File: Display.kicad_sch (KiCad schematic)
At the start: 0 parts

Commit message: Updated pin assignments
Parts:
- added DS1: HDSP-A22C, DIPS1524W51P254L2520H725Q18N, symbol UTSVT_LeaderSOM:HDSP-A22C
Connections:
- new net DISP_A: DS1.12 (1A/2A_CATHODE)
- new net DISP_B: DS1.10 (1B/2B_CATHODE)
- new net DISP_C: DS1.9 (1C/2C_CATHODE)
- new net DISP_D: DS1.7 (1D/2D_CATHODE)
- new net DISP_E: DS1.1 (1E/2E_CATHODE)
- new net DISP_F: DS1.18 (1F/2F_CATHODE)
- new net DISP_G: DS1.15 (1G/2G_CATHODE)
- new net DISP_H: DS1.14 (1H/2H_CATHODE)
- new net DISP_J: DS1.6 (1J/2J_CATHODE)
- new net DISP_K: DS1.5 (1K/2K_CATHODE)
- new net DISP_L: DS1.4 (1L/2L_CATHODE)
- new net DISP_M: DS1.2 (1M/2M_CATHODE)
- new net DISP_N: DS1.13 (1N/2N_CATHODE)
- new net DISP_P: DS1.17 (1P/2P_CATHODE)
- new net GND: DS1.11 (DIGIT_NO._2_COMMON_ANODE), DS1.16 (DIGIT_NO._1_COMMON_ANODE)
- no-connect marks 0 -> 2
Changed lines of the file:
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@@
 (kicad_sch (version 20230121) (generator eeschema)
   (paper "A4")
+  (no_connect (at 116.84 105.41))
+  (no_connect (at 116.84 92.71))
+  (wire (pts (xy 182.88 105.41) (xy 198.12 105.41))
+    (stroke (width 0) (type default))
+  )
+  (wire (pts (xy 182.88 92.71) (xy 198.12 92.71))
+    (stroke (width 0) (type default))
+  )
+  (wire (pts (xy 198.12 105.41) (xy 198.12 106.045))
+    (stroke (width 0) (type default))
+  )
+  (wire (pts (xy 198.12 92.71) (xy 198.12 93.345))
+    (stroke (width 0) (type default))
+  )
+  (hierarchical_label "DISP_J" (shape input) (at 116.84 100.33 180) (fields_autoplaced)
+    (effects (font (size 1.27 1.27)) (justify right))
+  )
+  (hierarchical_label "DISP_E" (shape input) (at 116.84 87.63 180) (fields_autoplaced)
+    (effects (font (size 1.27 1.27)) (justify right))
+  )
+  (hierarchical_label "DISP_F" (shape input) (at 182.88 87.63 0) (fields_autoplaced)
+    (effects (font (size 1.27 1.27)) (justify left))
+  )
+  (hierarchical_label "DISP_B" (shape input) (at 182.88 107.95 0) (fields_autoplaced)
+    (effects (font (size 1.27 1.27)) (justify left))
+  )
+  (hierarchical_label "DISP_H" (shape input) (at 182.88 97.79 0) (fields_autoplaced)
+    (effects (font (size 1.27 1.27)) (justify left))
+  )
+  (hierarchical_label "DISP_D" (shape input) (at 116.84 102.87 180) (fields_autoplaced)
+    (effects (font (size 1.27 1.27)) (justify right))
+  )
+  (hierarchical_label "DISP_M" (shape input) (at 116.84 90.17 180) (fields_autoplaced)
+    (effects (font (size 1.27 1.27)) (justify right))
+  )
+  (hierarchical_label "DISP_L" (shape input) (at 116.84 95.25 180) (fields_autoplaced)
+    (effects (font (size 1.27 1.27)) (justify right))
+  )
+  (hierarchical_label "DISP_G" (shape input) (at 182.88 95.25 0) (fields_autoplaced)
+    (effects (font (size 1.27 1.27)) (justify left))
+  )
+  (hierarchical_label "DISP_P" (shape input) (at 182.88 90.17 0) (fields_autoplaced)
+    (effects (font (size 1.27 1.27)) (justify left))
+  )
+  (hierarchical_label "DISP_C" (shape input) (at 116.84 107.95 180) (fields_autoplaced)
+    (effects (font (size 1.27 1.27)) (justify right))
+  )
+  (hierarchical_label "DISP_N" (shape input) (at 182.88 100.33 0) (fields_autoplaced)
+    (effects (font (size 1.27 1.27)) (justify left))
+  )
+  (hierarchical_label "DISP_A" (shape input) (at 182.88 102.87 0) (fields_autoplaced)
+    (effects (font (size 1.27 1.27)) (justify left))
+  )
+  (hierarchical_label "DISP_K" (shape input) (at 116.84 97.79 180) (fields_autoplaced)
+    (effects (font (size 1.27 1.27)) (justify right))
+  )
+  (symbol (lib_id "UTSVT_LeaderSOM:HDSP-A22C") (at 116.84 87.63 0) (unit 1)
+    (in_bom yes) (on_board yes) (dnp no)
+    (property "Reference" "DS1" (at 149.86 80.645 0)
+      (effects (font (size 1.27 1.27)))
+    )
+    (property "Value" "HDSP-A22C" (at 149.86 83.185 0)
+      (effects (font (size 1.27 1.27)))
+    )
+    (property "Footprint" "DIPS1524W51P254L2520H725Q18N" (at 179.07 182.55 0)
+      (effects (font (size 1.27 1.27)) (justify left top) hide)
+    )
+    (property "Datasheet" "https://docs.broadcom.com/docs/HDSP-A2xC-DS" (at 179.07 282.55 0)
+      (effects (font (size 1.27 1.27)) (justify left top) hide)
+    )
+    (property "Height" "7.25" (at 179.07 482.55 0)
+      (effects (font (size 1.27 1.27)) (justify left top) hide)
+    )
+    (property "Mouser Part Number" "630-HDSP-A22C" (at 179.07 582.55 0)
+      (effects (font (size 1.27 1.27)) (justify left top) hide)
+    )
+    (property "Mouser Price/Stock" "https://www.mouser.co.uk/ProductDetail/Broadcom-Avago/HDSP-A22C?qs=mhB89zxvawkE7eTk4oWrWQ%3D%3D" (at 179.07 682.55 0)
+      (effects (font (size 1.27 1.27)) (justify left top) hide)
+    )
+    (property "Manufacturer_Name" "Avago Technologies" (at 179.07 782.55 0)
+      (effects (font (size 1.27 1.27)) (justify left top) hide)
+    )
+    (property "Manufacturer_Part_Number" "HDSP-A22C" (at 179.07 882.55 0)
+      (effects (font (size 1.27 1.27)) (justify left top) hide)
+    )
+    (pin "1")
+    (pin "10")
+    (pin "11")
+    (pin "12")
+    (pin "13")
+    (pin "14")
+    (pin "15")
+    (pin "16")
+    (pin "17")
+    (pin "18")
+    (pin "2")
+    (pin "3")
+    (pin "4")
+    (pin "5")
+    (pin "6")
+    (pin "7")
+    (pin "8")
+    (pin "9")
+    (instances
+      (project "LeaderSOM"
+        (path "/192d0c36-944e-4927-949b-263b8c85a7ca/48d44a6a-93f2-4d40-b0ae-ce24d0554ae2"
+          (reference "DS1") (unit 1)
+        )
+      )
+    )
+  )
+  (symbol (lib_id "power:GND") (at 198.12 106.045 0) (unit 1)
+    (in_bom yes) (on_board yes) (dnp no)
+    (property "Reference" "#PWR021" (at 198.12 112.395 0)
+      (effects (font (size 1.27 1.27)) hide)
+    )
+    (property "Value" "GND" (at 198.247 110.4392 0)
+      (effects (font (size 1.27 1.27)))
+    )
+    (property "Footprint" "" (at 198.12 106.045 0)
+      (effects (font (size 1.27 1.27)) hide)
+    )
+    (property "Datasheet" "" (at 198.12 106.045 0)
+      (effects (font (size 1.27 1.27)) hide)
+    )
+    (pin "1")
+    (instances
+      (project "LeaderSOM"
+        (path "/192d0c36-944e-4927-949b-263b8c85a7ca"
+          (reference "#PWR021") (unit 1)
+        )
+        (path "/192d0c36-944e-4927-949b-263b8c85a7ca/48d44a6a-93f2-4d40-b0ae-ce24d0554ae2"
+          (reference "#PWR027") (unit 1)
+        )
+      )
+      (project "BPS-Leader"
+        (path "/c248b171-df31-4e8a-afb6-607fa2df334b"
+          (reference "#PWR08") (unit 1)
+        )
+      )
+    )
+  )
+  (symbol (lib_id "power:GND") (at 198.12 93.345 0) (unit 1)
+    (in_bom yes) (on_board yes) (dnp no)
+    (property "Reference" "#PWR021" (at 198.12 99.695 0)
+      (effects (font (size 1.27 1.27)) hide)
+    )
+    (property "Value" "GND" (at 198.247 97.7392 0)
+      (effects (font (size 1.27 1.27)))
+    )
+    (property "Footprint" "" (at 198.12 93.345 0)
+      (effects (font (size 1.27 1.27)) hide)
+    )
+    (property "Datasheet" "" (at 198.12 93.345 0)
+      (effects (font (size 1.27 1.27)) hide)
+    )
+    (pin "1")
+    (instances
+      (project "LeaderSOM"
+        (path "/192d0c36-944e-4927-949b-263b8c85a7ca"
+          (reference "#PWR021") (unit 1)
+        )
+        (path "/192d0c36-944e-4927-949b-263b8c85a7ca/48d44a6a-93f2-4d40-b0ae-ce24d0554ae2"
+          (reference "#PWR028") (unit 1)
+        )
+      )
+      (project "BPS-Leader"
+        (path "/c248b171-df31-4e8a-afb6-607fa2df334b"
+          (reference "#PWR08") (unit 1)
+        )
+      )
+    )
+  )
 )

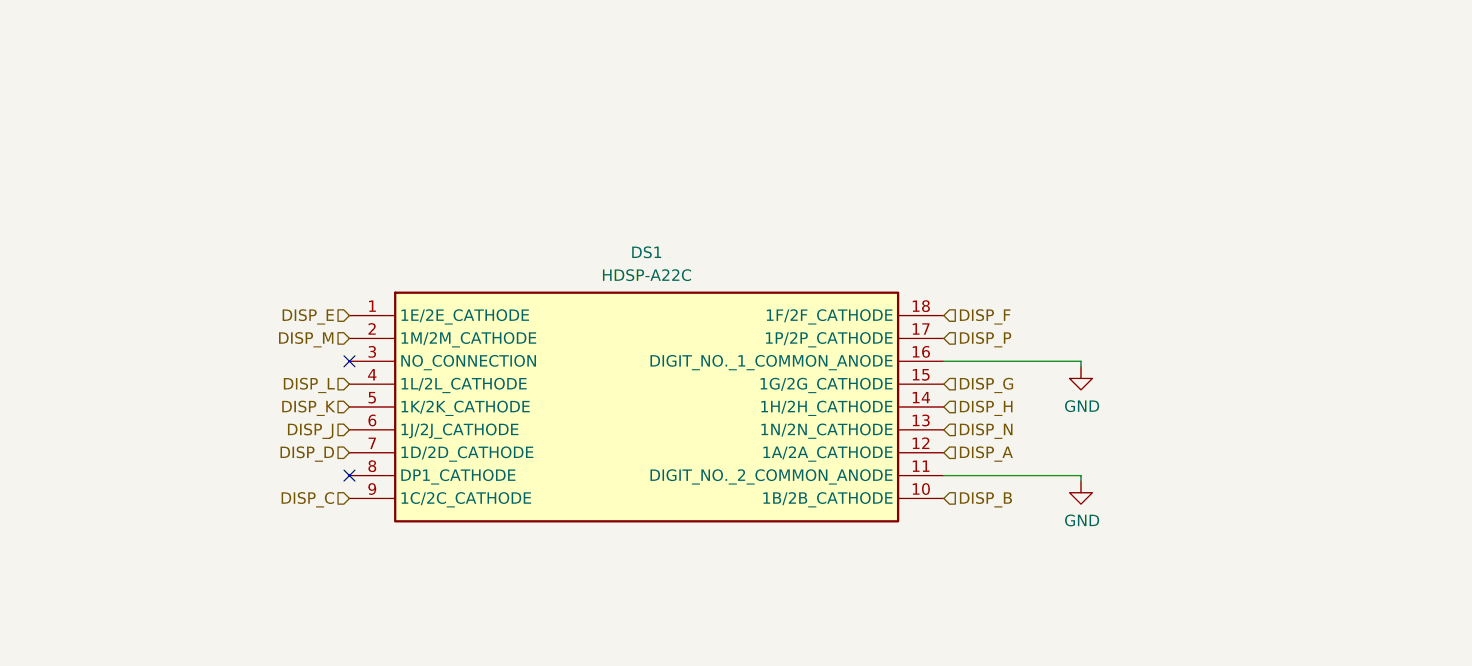
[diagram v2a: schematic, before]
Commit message: Updated power dist and CAN circuitry
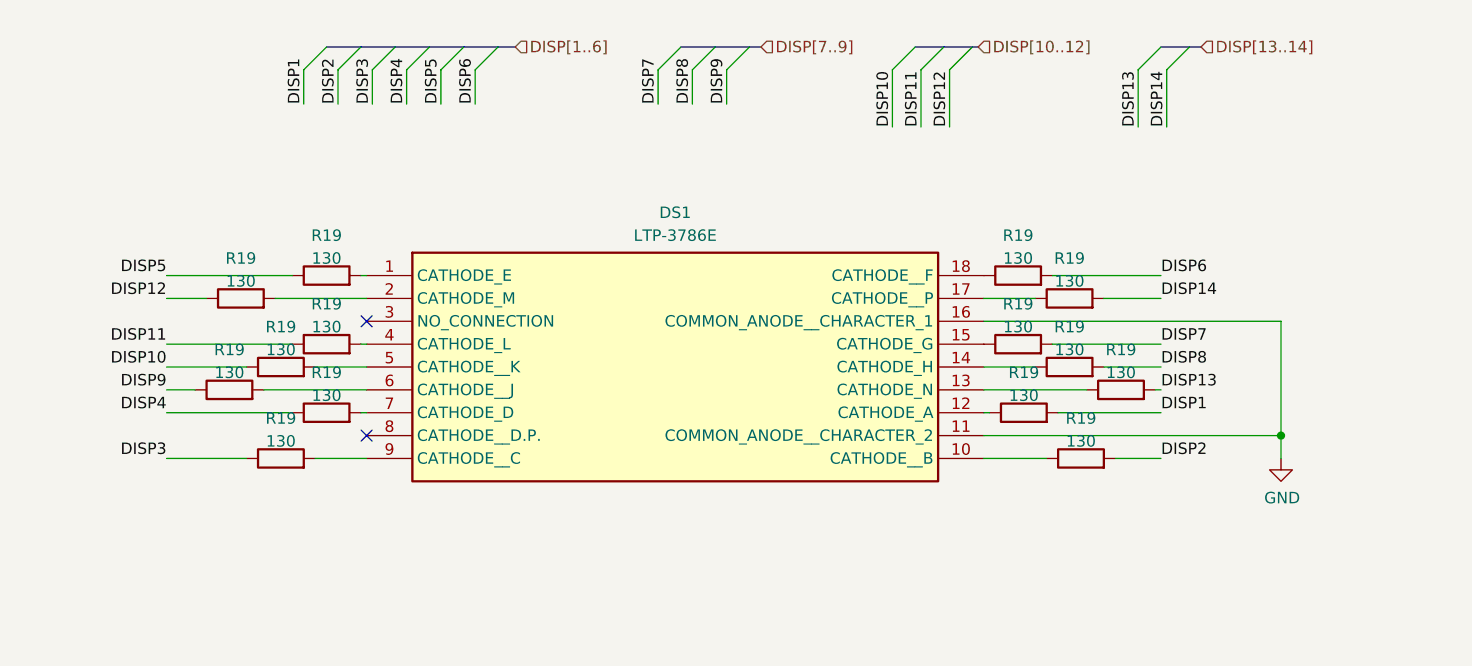
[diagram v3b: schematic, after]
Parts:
- removed DS1: HDSP-A22C, DIPS1524W51P254L2520H725Q18N, symbol UTSVT_LeaderSOM:HDSP-A22C
- added DS1: LTP-3786E, DIPS1499W50P254L2520H805Q18N, symbol UTSVT_LeaderSOM:LTP-3786E
- added R19 (x14): 130, Resistor_SMD:R_0805_2012Metric, symbol Device:R
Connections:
- net GND: now also DS1.11 (COMMON_ANODE__CHARACTER_2), DS1.16 (COMMON_ANODE__CHARACTER_1)
- new net: DS1.10 (CATHODE__B), R19.1
- new net: DS1.4 (CATHODE_L), R19.2
- new net: DS1.15 (CATHODE_G), R19.1
- new net: DS1.18 (CATHODE__F), R19.1
- new net: DS1.1 (CATHODE_E), R19.2
- new net: DS1.12 (CATHODE_A), R19.1
- new net: DS1.13 (CATHODE_N), R19.1
- new net: DS1.14 (CATHODE_H), R19.1
- new net: DS1.17 (CATHODE__P), R19.1
- new net: DS1.2 (CATHODE_M), R19.2
- new net: DS1.5 (CATHODE__K), R19.2
- new net: DS1.6 (CATHODE__J), R19.2
- new net: DS1.7 (CATHODE_D), R19.2
- new net: DS1.9 (CATHODE__C), R19.2
- new net DISP1: R19.2
- new net DISP10: R19.1
- new net DISP11: R19.1
- new net DISP12: R19.1
- new net DISP13: R19.2
- new net DISP14: R19.2
- new net DISP2: R19.2
- new net DISP3: R19.1
- new net DISP4: R19.1
- new net DISP5: R19.1
- new net DISP6: R19.2
- new net DISP7: R19.2
- new net DISP8: R19.2
- new net DISP9: R19.1

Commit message: Updated symbols
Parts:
- removed DS1: LTP-3786E, DIPS1499W50P254L2520H805Q18N, symbol UTSVT_LeaderSOM:LTP-3786E
- added DS1: LTP-3786E, DIPS1499W50P254L2520H805Q18N, symbol utsvt-misc:LTP-3786E
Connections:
- net GND: now also DS1.11 (COMMON_ANODE__CHARACTER_2), DS1.16 (COMMON_ANODE__CHARACTER_1)
- net at R19.1: now also DS1.10 (CATHODE__B)
- net at R19.2: now also DS1.4 (CATHODE_L)
- net at R19.1: now also DS1.15 (CATHODE_G)
- net at R19.1: now also DS1.18 (CATHODE__F)
- net at R19.2: now also DS1.1 (CATHODE_E)
- net at R19.1: now also DS1.12 (CATHODE_A)
- net at R19.1: now also DS1.13 (CATHODE_N)
- net at R19.1: now also DS1.14 (CATHODE_H)
- net at R19.1: now also DS1.17 (CATHODE__P)
- net at R19.2: now also DS1.2 (CATHODE_M)
- net at R19.2: now also DS1.5 (CATHODE__K)
- net at R19.2: now also DS1.6 (CATHODE__J)
- net at R19.2: now also DS1.7 (CATHODE_D)
- net at R19.2: now also DS1.9 (CATHODE__C)

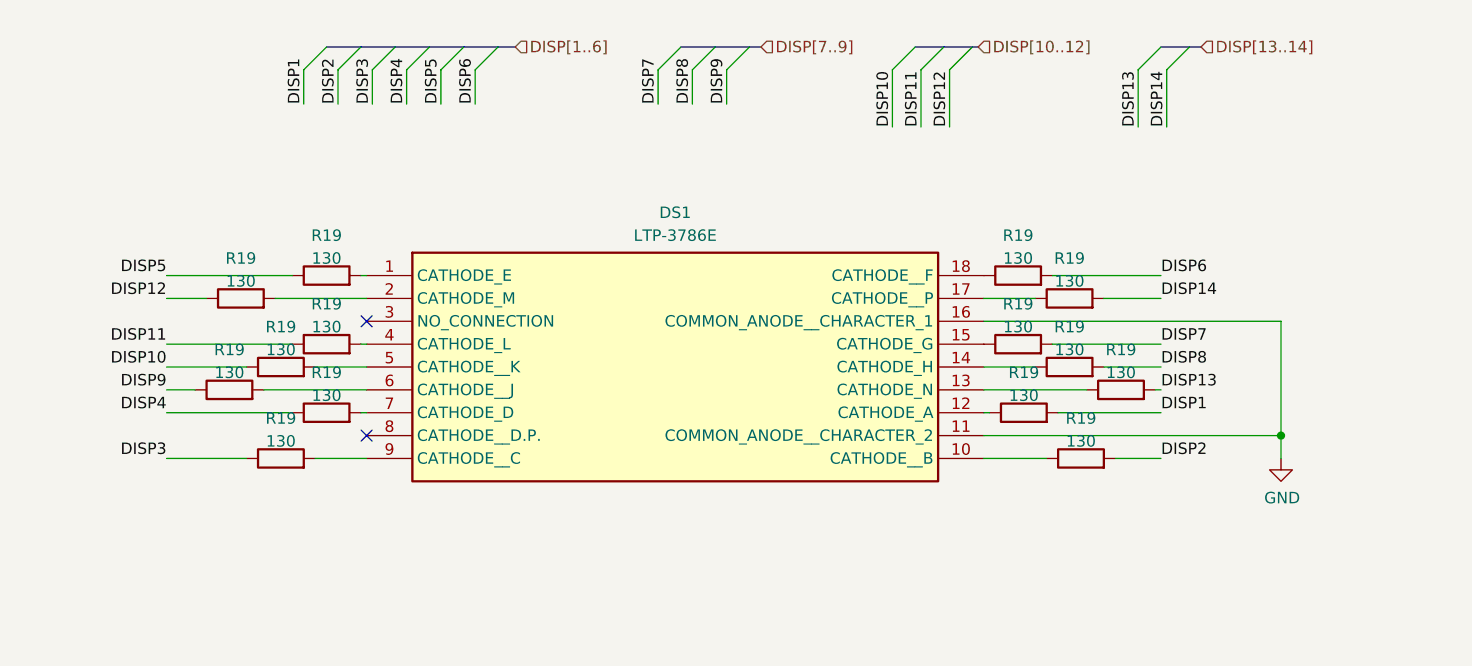
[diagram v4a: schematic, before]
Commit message: a
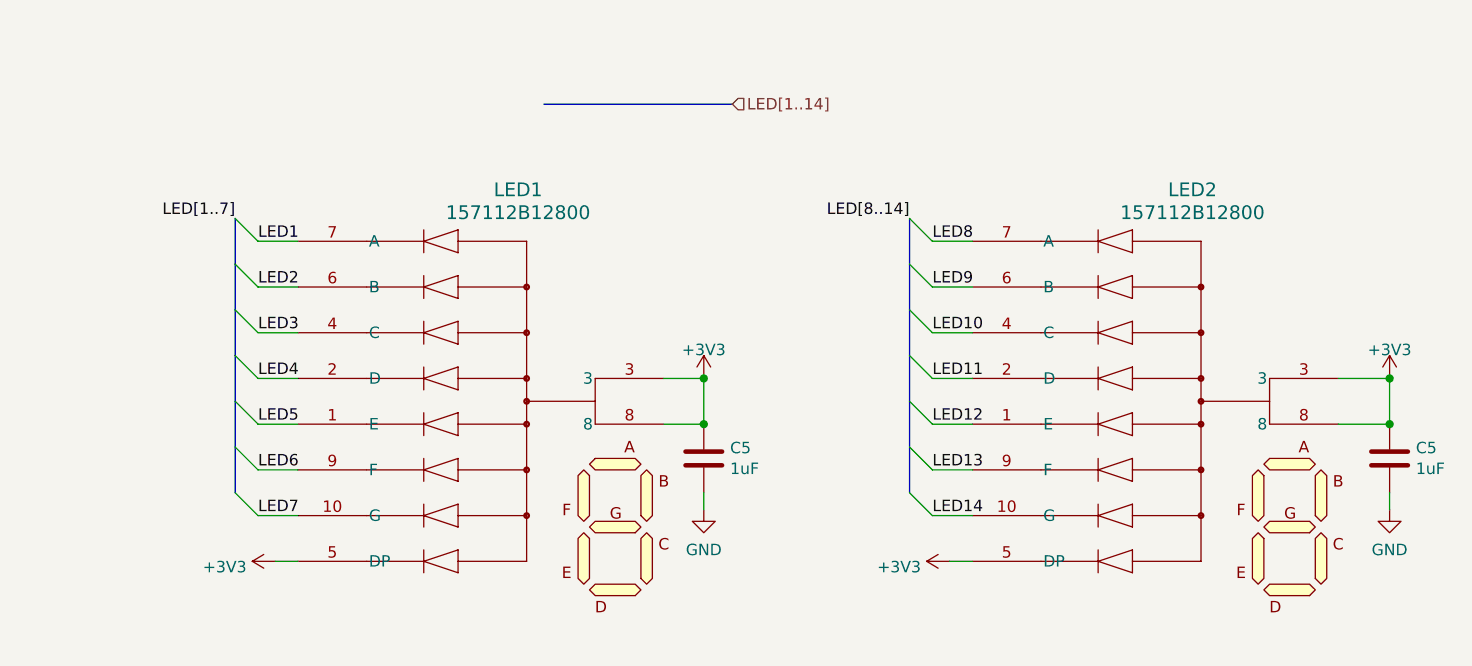
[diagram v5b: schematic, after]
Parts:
- removed DS1: LTP-3786E, DIPS1499W50P254L2520H805Q18N, symbol utsvt-misc:LTP-3786E
- removed R19 (x14): 130, Resistor_SMD:R_0805_2012Metric, symbol Device:R
- added C5 (x2): 1uF, Capacitor_SMD:C_0805_2012Metric, symbol Device:C
- added LED1, LED2: 157112B12800, UTSVT_Special:SMT_1S12800_WRE, symbol utsvt-misc:157112B12800
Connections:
- net GND: now also C5.2, C5.2
- new net +3V3: C5.1, C5.1, LED1.3, LED1.5 (DP), LED1.8, LED2.3, LED2.5 (DP), LED2.8
- new net LED1: LED1.7 (A)
- new net LED10: LED2.4 (C)
- new net LED11: LED2.2 (D)
- new net LED12: LED2.1 (E)
- new net LED13: LED2.9 (F)
- new net LED14: LED2.10 (G)
- new net LED2: LED1.6 (B)
- new net LED3: LED1.4 (C)
- new net LED4: LED1.2 (D)
- new net LED5: LED1.1 (E)
- new net LED6: LED1.9 (F)
- new net LED7: LED1.10 (G)
- new net LED8: LED2.7 (A)
- new net LED9: LED2.6 (B)
- no-connect marks 2 -> 0

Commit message: updated pin assignments
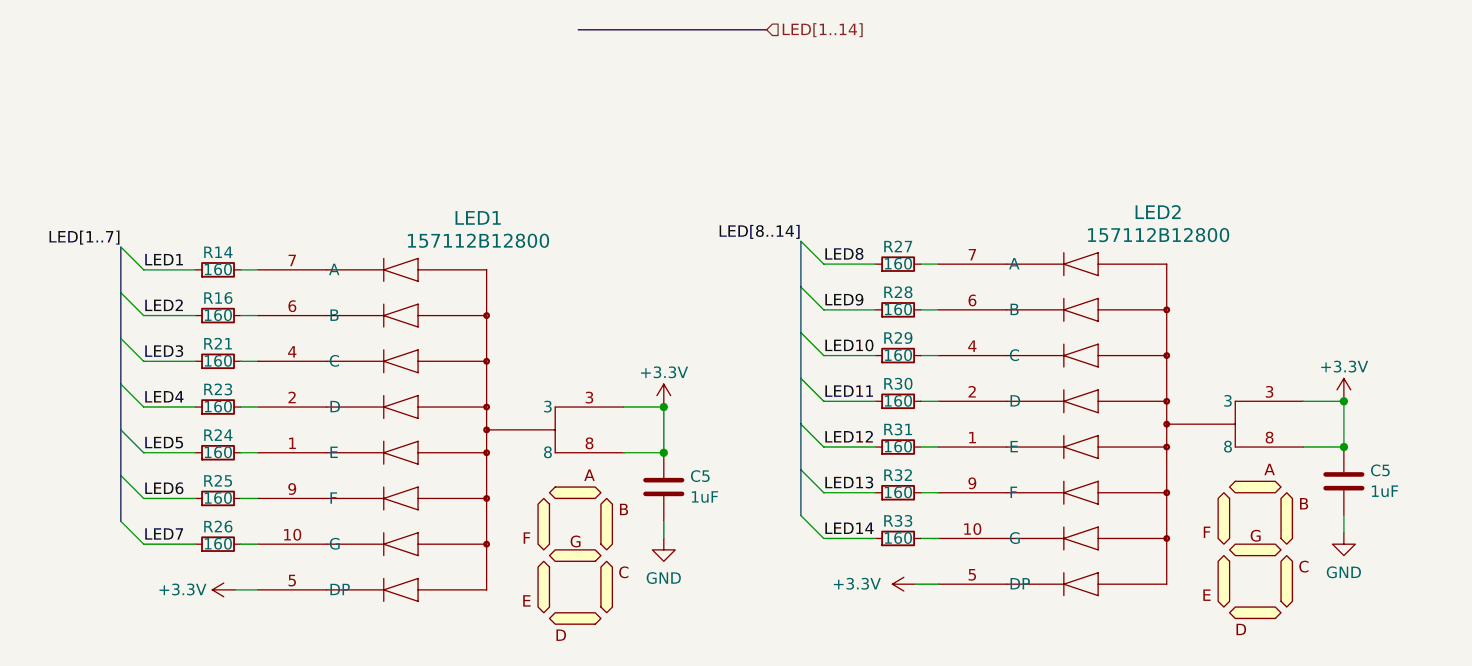
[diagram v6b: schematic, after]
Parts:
- added R14, R16, R21, R23, R24, R25, R26, R27, R28, R29, R30, R31, R32, R33: 160, Resistor_SMD:R_0805_2012Metric, symbol Device:R_Small
- LED1, LED2: P/N (none) -> 157112B12800
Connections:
- net LED1: now also R14.1; no longer LED1.7 (A)
- net LED10: now also R29.1; no longer LED2.4 (C)
- net LED11: now also R30.1; no longer LED2.2 (D)
- net LED12: now also R31.1; no longer LED2.1 (E)
- net LED13: now also R32.1; no longer LED2.9 (F)
- net LED14: now also R33.1; no longer LED2.10 (G)
- net LED2: now also R16.1; no longer LED1.6 (B)
- net LED3: now also R21.1; no longer LED1.4 (C)
- net LED4: now also R23.1; no longer LED1.2 (D)
- net LED5: now also R24.1; no longer LED1.1 (E)
- net LED6: now also R25.1; no longer LED1.9 (F)
- net LED7: now also R26.1; no longer LED1.10 (G)
- net LED8: now also R27.1; no longer LED2.7 (A)
- net LED9: now also R28.1; no longer LED2.6 (B)
- net +3V3 renamed +3.3V
- new net: LED2.1 (E), R31.2
- new net: LED2.10 (G), R33.2
- new net: LED2.2 (D), R30.2
- new net: LED2.4 (C), R29.2
- new net: LED2.6 (B), R28.2
- new net: LED2.7 (A), R27.2
- new net: LED2.9 (F), R32.2
- new net: LED1.6 (B), R16.2
- new net: LED1.2 (D), R23.2
- new net: LED1.4 (C), R21.2
- new net: LED1.9 (F), R25.2
- new net: LED1.7 (A), R14.2
- new net: LED1.1 (E), R24.2
- new net: LED1.10 (G), R26.2
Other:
- moved on the sheet: C5
